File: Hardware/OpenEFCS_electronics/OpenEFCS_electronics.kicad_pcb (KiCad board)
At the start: 2 copper layers, 88 x 17 mm, 68 parts, among them J1 15v, J2 GND, J3 M+, J4 M-, J5 CTRL-B, J6 PGRM, J7 CTRL-F, Q1 DMG3402L, Q2 BSC010N04LS6, Q3 BSC010N04LS6, SW1 DECOCK, U1 STM32F042K4Tx, U2 AP1117-33, U3 BL9342, U4 XJNG2103, U5 INA2180A4, Y1 8MHz 12pF

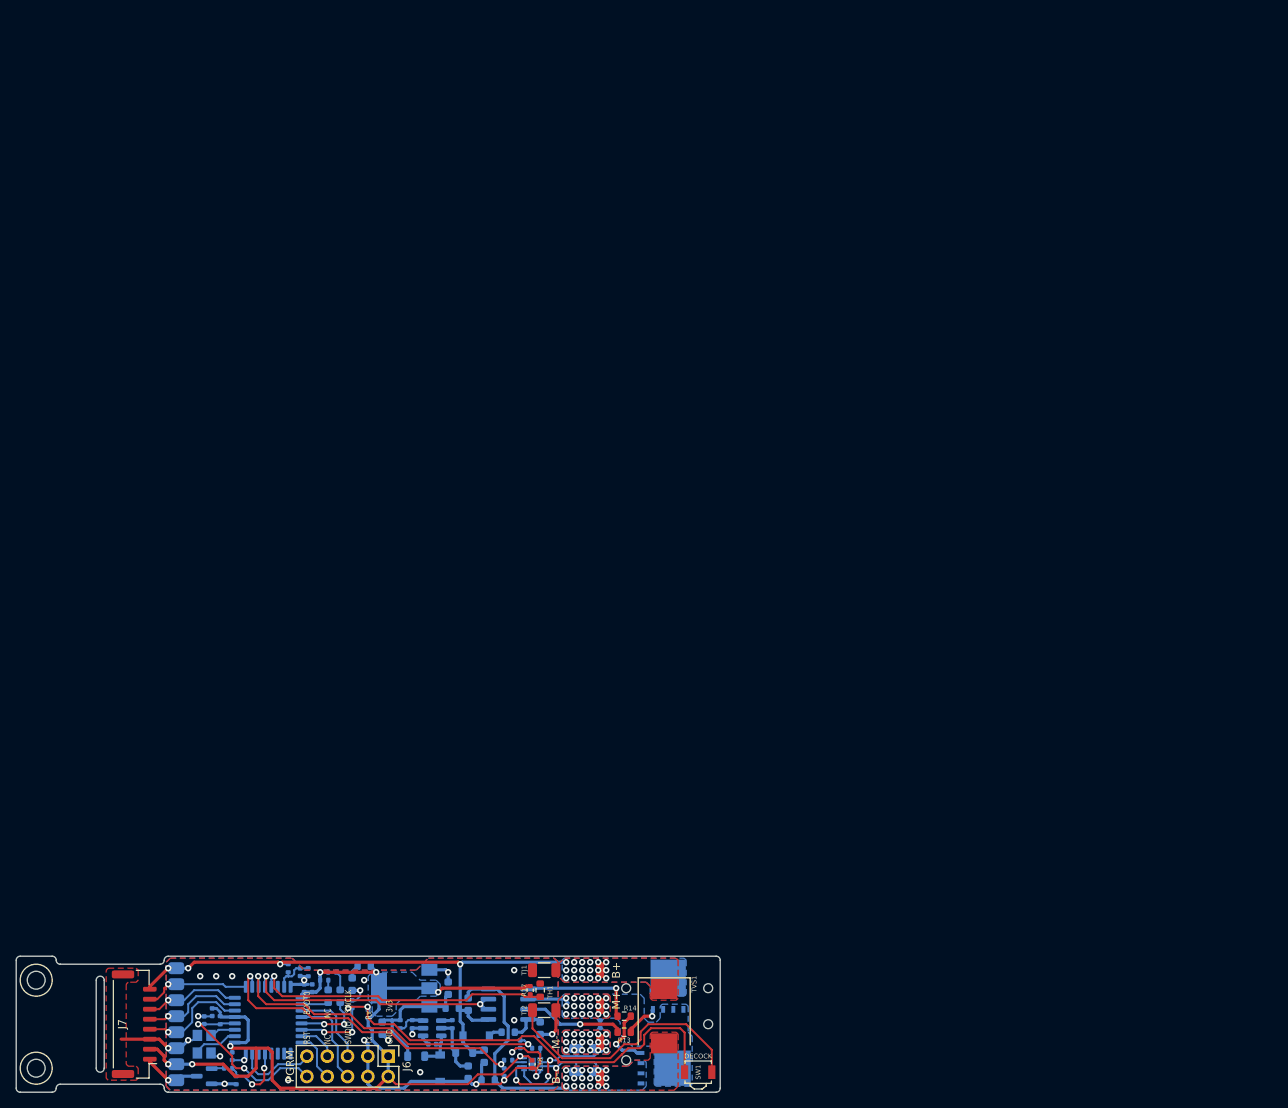
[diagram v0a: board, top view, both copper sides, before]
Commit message: design complete for second prototype
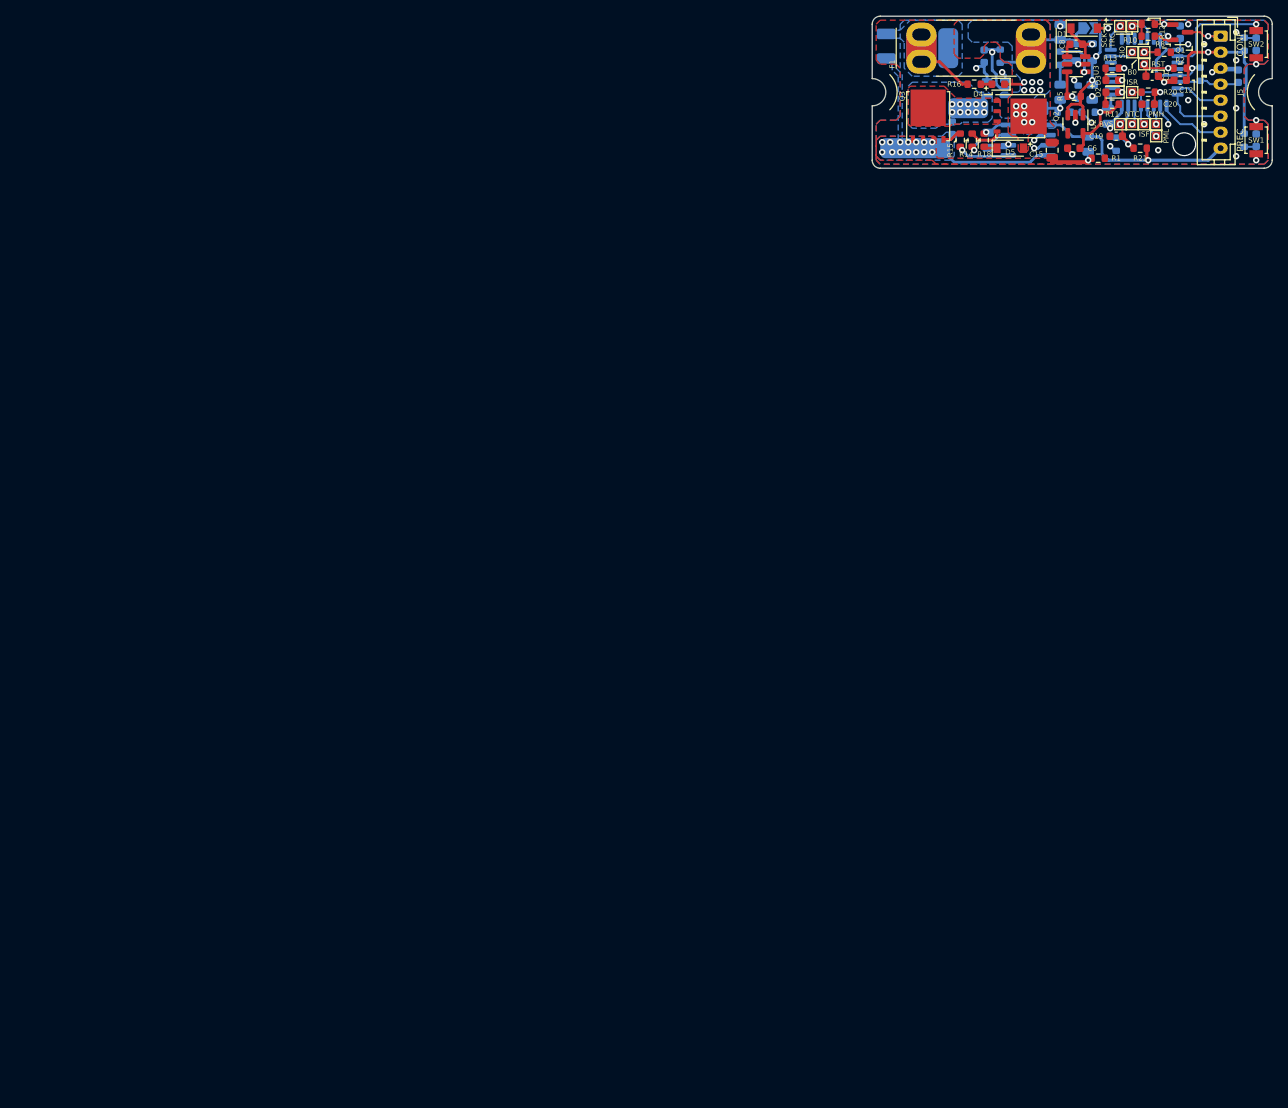
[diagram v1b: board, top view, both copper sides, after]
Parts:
- removed C5: 22u, Capacitor_SMD:C_0603_1608Metric
- removed J6: PGRM, Connector_PinHeader_2.54mm:PinHeader_2x05_P2.54mm_Vertical
- removed J7: CTRL-F, Connector_JST:JST_GH_BM08B-GHS-TBT_1x08-1MP_P1.25mm_Vertical
- removed Ris1, Ris2: 0.5m, Resistor_SMD:R_1206_3216Metric
- removed TJ2: Thermal Jumper, Resistor_SMD:R_1206_3216Metric
- removed TVS1: SMDJ15A-HR, Diode_SMD:D_SMC
- removed Y1: 8MHz 12pF, Crystal:Crystal_SMD_3225-4Pin_3.2x2.5mm
- added C20: 100n, Capacitor_SMD:C_0603_1608Metric, F.Cu at (168.5, -15.5)
- added CIN1: 22uF, Capacitor_Tantalum_SMD:CP_EIA-3528-12_Kemet-T, B.Cu at (135.8, -22.8)
- added D5: GOODWORK K14, Diode_SMD:D_SOD-123, F.Cu at (151.2, -10.0)
- added F1: 3557, KiCAD-Custom-Lib:Keystone 3557, F.Cu at (147.0, -22.5)
- added JP1: BYP, Jumper:SolderJumper-2_P1.3mm_Open_TrianglePad1.0x1.5mm, B.Cu at (161.0, -25.0)
- added R21: 56k, Resistor_SMD:R_0603_1608Metric, F.Cu at (167.5, -10.0)
- added R22: 10k, Resistor_SMD:R_0603_1608Metric, B.Cu at (164.5, -10.5)
- added SW2: CONF, Button_Switch_SMD:SW_SPST_B3U-1000P, F.Cu at (182.0, -23.0)
- added TP1: NTC, TestPoint:TestPoint_Pad_1.0x1.0mm, F.Cu at (166.5, -13.0)
- added TP10: BVS, TestPoint:TestPoint_Pad_1.0x1.0mm, F.Cu at (165.0, -13.0)
- added TP11: ISF, TestPoint:TestPoint_Pad_1.0x1.0mm, F.Cu at (168.0, -13.0)
- added TP2: PML, TestPoint:TestPoint_Pad_1.0x1.0mm, F.Cu at (169.5, -11.5)
- added TP3: PMH, TestPoint:TestPoint_Pad_1.0x1.0mm, F.Cu at (169.5, -13.0)
- added TP4: TRC, TestPoint:TestPoint_Pad_1.0x1.0mm, F.Cu at (166.5, -25.2)
- added TP5: ISR, TestPoint:TestPoint_Pad_1.0x1.0mm, F.Cu at (166.5, -17.0)
- added TP6: SIO, TestPoint:TestPoint_Pad_1.0x1.0mm, F.Cu at (166.5, -22.0)
- added TP7: B0, TestPoint:TestPoint_Pad_1.0x1.0mm, F.Cu at (168.0, -22.0)
- added TP8: RST, TestPoint:TestPoint_Pad_1.0x1.0mm, F.Cu at (168.0, -20.5)
- added TP9: SCK, TestPoint:TestPoint_Pad_1.0x1.0mm, F.Cu at (165.0, -25.2)
- C1, C19, C6, C8: footprint Capacitor_SMD:C_0402_1005Metric -> Capacitor_SMD:C_0603_1608Metric; moved to F.Cu
- C10, C13, C16, C17: value 100n -> 10u; footprint Capacitor_SMD:C_0402_1005Metric -> Capacitor_SMD:C_0805_2012Metric
- C11, C7: footprint Capacitor_SMD:C_0402_1005Metric -> Capacitor_SMD:C_0603_1608Metric
- C12: value 4.7u -> 100n; footprint Capacitor_SMD:C_0402_1005Metric -> Capacitor_SMD:C_0603_1608Metric; moved to F.Cu
- C14, C3: value 10u -> 100n
- C15: footprint Capacitor_SMD:C_0603_1608Metric -> Capacitor_SMD:C_0805_2012Metric; moved to F.Cu
- C18: footprint Capacitor_SMD:C_0402_1005Metric -> Capacitor_SMD:C_0603_1608Metric; moved to B.Cu
- C2, C4: footprint Capacitor_SMD:C_0603_1608Metric -> Capacitor_SMD:C_0805_2012Metric
- C9: value 22u -> 100n
- D1, D2, D3, Q1, Q2, Q3, R1, R15, U3: moved to F.Cu
- D4: value GOODWORK K14 -> YLW; footprint Diode_SMD:D_SOD-123 -> LED_SMD:LED_0603_1608Metric; moved to F.Cu
- J1, J2, J3, J4, TH1: moved to B.Cu
- J5: value CTRL-B -> CTRL; footprint Connector_PinHeader_2.00mm:PinHeader_1x08_P2.00mm_Vertical -> Connector_JST:JST_PH_B8B-PH-K_1x08_P2.00mm_Vertical; moved to F.Cu
- L1, L2: value 10uH -> 6.8uH
- R10: value 1.5k -> 56k; footprint Resistor_SMD:R_0402_1005Metric -> Resistor_SMD:R_0603_1608Metric; moved to F.Cu
- R11, R12, R16, R5: footprint Resistor_SMD:R_0402_1005Metric -> Resistor_SMD:R_0603_1608Metric; moved to F.Cu
- R13: value 1R8 -> 1.5k
- R17: value 1.5k -> 10k; footprint Resistor_SMD:R_0402_1005Metric -> Resistor_SMD:R_0603_1608Metric; moved to B.Cu
- R18: value 1.5k -> 1R8; footprint Resistor_SMD:R_0402_1005Metric -> Resistor_SMD:R_0603_1608Metric; moved to F.Cu
- R19: value 56k -> 1.5k; footprint Resistor_SMD:R_0402_1005Metric -> Resistor_SMD:R_0603_1608Metric
- R2: value 10k -> 56k; footprint Resistor_SMD:R_0402_1005Metric -> Resistor_SMD:R_0603_1608Metric; moved to F.Cu
- R20: value 10k -> 1.5k; footprint Resistor_SMD:R_0402_1005Metric -> Resistor_SMD:R_0603_1608Metric; moved to F.Cu
- R3, R6, R7: footprint Resistor_SMD:R_0402_1005Metric -> Resistor_SMD:R_0603_1608Metric
- R4: value 1R8 -> 10k
- R8: value 0 -> 56k; moved to F.Cu
- R9: value 56k -> 10k; footprint Resistor_SMD:R_0402_1005Metric -> Resistor_SMD:R_0603_1608Metric
- SW1: value DECOCK -> PREC; footprint Button_Switch_SMD:SW_SPST_B3U-3000P -> Button_Switch_SMD:SW_SPST_B3U-1000P
- TJ1: value Thermal Jumper -> ThermJmpr; moved to B.Cu
- U2: value AP1117-33 -> AP2204K-3.3; footprint Package_TO_SOT_SMD:SOT-223-3_TabPin2 -> Package_TO_SOT_SMD:SOT-23-5; moved to F.Cu
- U5: value INA2180A4 -> INA194; footprint Package_DFN_QFN:DFN-8-1EP_2x2mm_P0.5mm_EP0.9x1.6mm -> Package_TO_SOT_SMD:SOT-23-5
- moved J5 184.6 mm to (177.6, -24.0), turned to -90 degrees
- moved R9 180.7 mm to (180.5, -23.0), turned to -90 degrees
- moved Q1 178.6 mm to (172.5, -24.5), turned to 0 degrees
- moved R2 169.0 mm to (172.5, -20.0), turned to 0 degrees
- moved C11 167.6 mm to (182.0, -23.0), turned to -90 degrees
- moved C1 167.2 mm to (169.0, -19.0), turned to 0 degrees
- moved R11 163.5 mm to (164.0, -15.5)
- moved C8 162.2 mm to (159.5, -23.0), turned to 0 degrees
- moved U1 161.3 mm to (168.0, -19.5), turned to 180 degrees
- moved C9 159.5 mm to (172.5, -24.5), turned to 90 degrees
- moved C3 157.4 mm to (179.8, -19.0), turned to 90 degrees
- moved C12 157.0 mm to (172.5, -18.5), turned to 180 degrees
- moved R10 156.6 mm to (168.5, -24.0)
- moved R12 156.4 mm to (168.5, -25.5)
- moved C6 154.8 mm to (159.2, -10.0), turned to 180 degrees
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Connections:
- C10 pad 1: /DECOCK -> +5V
- C11 pad 1: +3V3 -> /CONF
- C13 pad 1: /M+ -> +3V3
- C13 pad 2: /ISENSE_RAW -> GNDREF
- C14 pad 1: +15V -> /M+
- C15 pad 1: /M+ -> +15V
- C15 pad 2: Net-(C15-Pad2) -> GNDPWR
- C16 pad 1: /ISENSE_BRAKE_LP -> +15V
- C16 pad 2: GNDREF -> GNDPWR
- C17 pad 1: /BATT_SENSE -> /M+
- C17 pad 2: GNDREF -> Net-(C17-Pad2)
- C18 pad 1: +3V3 -> GNDREF
- C18 pad 2: GNDREF -> +3V3
- C19 pad 1: /ISENSE_RUN_LP -> /BATT_SENSE
- C3 pad 1: Net-(C3-Pad1) -> /AIN1
- C4 pad 1: +5V -> Net-(C4-Pad1)
- C7 pad 1: Net-(C7-Pad1) -> /PREC
- C7 pad 2: Net-(C7-Pad2) -> GNDREF
- C8 pad 1: +3V3 -> Net-(C8-Pad1)
- C8 pad 2: GNDREF -> Net-(C8-Pad2)
- C9 pad 1: +5V -> +3V3
- D1 pad 1: Net-(C7-Pad2) -> Net-(C8-Pad2)
- D4 pad 1: Net-(D4-Pad1) -> +15V
- D4 pad 2: +15V -> Net-(D4-Pad2)
- J1 pad 1: +15V -> +BATT
- J4 pad 1: /ISENSE_RAW -> GNDPWR
- L1 pad 2: Net-(C3-Pad1) -> Net-(C4-Pad1)
- L2 pad 1: Net-(C7-Pad2) -> Net-(C8-Pad2)
- R10 pad 1: Net-(D2-Pad2) -> GNDREF
- R10 pad 2: +3V3 -> /Tracer
- R11 pad 1: Net-(Q1-Pad1) -> Net-(D2-Pad2)
- R11 pad 2: /Tracer -> +3V3
- R12 pad 1: Net-(D3-Pad2) -> Net-(Q1-Pad1)
- R12 pad 2: +3V3 -> /Tracer
- R13 pad 1: Net-(Q2-Pad4) -> Net-(D3-Pad2)
- R13 pad 2: /HB_HIGH -> +3V3
- R14 pad 1: Net-(Q3-Pad4) -> Net-(Q2-Pad4)
- R14 pad 2: /HB_LOW -> /HB_HIGH
- R15 pad 1: Net-(C15-Pad2) -> Net-(Q3-Pad4)
- R15 pad 2: Net-(D4-Pad1) -> /HB_LOW
- R16 pad 1: /ISENSE_BRAKE_LP -> +BATT
- R16 pad 2: /ISENSE_BRAKE -> Net-(D4-Pad2)
- R17 pad 1: /NTC -> GNDREF
- R17 pad 2: +3V3 -> +15V
- R18 pad 1: /ISENSE_RUN_LP -> Net-(C17-Pad2)
- R18 pad 2: /ISENSE_RUN -> Net-(D5-Pad1)
- R19 pad 1: /BATT_SENSE -> /NTC
- R19 pad 2: +15V -> +3V3
- R20 pad 1: GNDREF -> /ISENSE_RUN_LP
- R20 pad 2: /BATT_SENSE -> /ISENSE_RUN
- R3 pad 1: Net-(R3-Pad1) -> /AIN1
- R3 pad 2: Net-(C3-Pad1) -> +3V3
- R4 pad 1: Net-(C5-Pad1) -> Net-(R4-Pad1)
- R4 pad 2: +3V3 -> Net-(C4-Pad1)
- R7 pad 1: /DECOCK -> /PREC
- R8 pad 1: +5V -> GNDREF
- R8 pad 2: +15V -> /BOOT0
- R9 pad 1: GNDREF -> /CONF
- R9 pad 2: /Tracer -> +3V3
- SW1 pad 2: /DECOCK -> /PREC
- U1 pad 10: /ISENSE_RUN_LP -> /PREC
- U1 pad 11: /ISENSE_BRAKE_LP -> /PWMH
- U1 pad 12: /PWMMOT -> /PWML
- U1 pad 13: /NTC -> /ISENSE_RUN_LP
- U1 pad 14: unconnected-(U1-Pad14) -> /NTC
- U1 pad 19: /Tx -> /LED1
- U1 pad 2: /OSCIN -> /CONF
- U1 pad 20: /Rx -> unconnected-(U1-Pad20)
- U1 pad 21: /LED1 -> unconnected-(U1-Pad21)
- U1 pad 22: /DECOCK -> unconnected-(U1-Pad22)
- U1 pad 3: /OSCOUT -> unconnected-(U1-Pad3)
- U2 pad 1: GNDREF -> +5V
- U2 pad 2: +3V3 -> GNDREF
- U3 pad 1: Net-(C7-Pad1) -> Net-(C8-Pad1)
- U3 pad 4: Net-(R3-Pad1) -> Net-(R4-Pad1)
- U3 pad 5: Net-(C3-Pad1) -> Net-(C4-Pad1)
- U3 pad 6: Net-(C7-Pad2) -> Net-(C8-Pad2)
- U4 pad 2: /PWMMOT -> /PWMH
- U4 pad 3: /PWMMOT -> /PWML
- U4 pad 8: Net-(C15-Pad2) -> Net-(C17-Pad2)
- U5 pad 1: /ISENSE_BRAKE -> /ISENSE_RUN
- U5 pad 2: /ISENSE_RAW -> GNDREF
- U5 pad 3: GNDPWR -> +15V
- U5 pad 4: GNDREF -> /M+
- U5 pad 5: /ISENSE_RAW -> +3V3
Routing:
- net +3V3: track 123.0 -> 50.7 mm, vias 7 -> 5
- net GNDREF: track 109.5 -> 41.8 mm, vias 24 -> 26
- net /DECOCK: track 64.0 -> 0.00 mm, vias 4 -> 0
- net /ISENSE_BRAKE_LP: track 42.0 -> 0.00 mm, vias 2 -> 0
- net /PWMMOT: track 33.3 -> 0.00 mm, vias 2 -> 0
- net /ISENSE_RUN_LP: track 40.1 -> 8.53 mm
- net +15V: track 72.8 -> 42.9 mm, vias 22 -> 13
- net /NTC: track 37.6 -> 12.5 mm, vias 1 -> 2
- net /PWML: track 0.00 -> 23.3 mm, vias 0 -> 2
- net /PREC: track 0.00 -> 22.6 mm, vias 0 -> 2
- net /PWMH: track 0.00 -> 22.6 mm, vias 0 -> 2
- net GNDPWR: track 45.9 -> 23.5 mm, vias 20 -> 15
- net /ISENSE_RUN: track 1.58 -> 22.4 mm, vias 0 -> 2
- net /CONF: track 0.00 -> 17.3 mm, vias 0 -> 1
- net /ISENSE_RAW: track 16.0 -> 0.00 mm, vias 20 -> 0
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- added copper zone on In1.Cu, net +15V
- added copper zone on In2.Cu, net +15V
- added copper zone on In1.Cu, net +3V3
- added copper zone on B.Cu, net +BATT
- added copper zone on In1.Cu, net /M+
- added copper zone on In2.Cu, net /M+
- added copper zone on In2.Cu, net GNDREF
- removed copper zone on B.Cu, net +3V3
- removed copper zone on B.Cu, net /ISENSE_RAW
- removed copper zone on F.Cu, net /ISENSE_RAW
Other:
- board size 88 x 17 mm -> 50 x 19 mm
- copper layers 2 -> 4
- board text added: "15v"
- board text added: "3v3 GND"
- board text added: "B0"
- board text added: "BVS"
- board text added: "CONF"
- board text added: "ISF"
- board text added: "ISR"
- board text added: "NTC"
- board text added: "PGND"
- board text added: "PMH"
- board text added: "PML"
- board text added: "PREC"
- board text added: "RST"
- board text added: "SCK"
- board text added: "SIO"
- board text added: "TCR-"
- board text added: "TRC"
- board text added: "TRG AIN Tx Rx"
- board text removed: "B-"
- board text removed: "M-"
- board text removed: "RST BOOT0 NC NC SWDIO SWCLK Tx Rx GND 3v3"
